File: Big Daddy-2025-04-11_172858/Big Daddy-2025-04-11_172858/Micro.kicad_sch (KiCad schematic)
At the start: 22 parts, among them Q1 2N7002, U1 MAX33054EASA+T, U2 ESP32-S3-DevKitC, U3 ESP32-S3-DevKitC

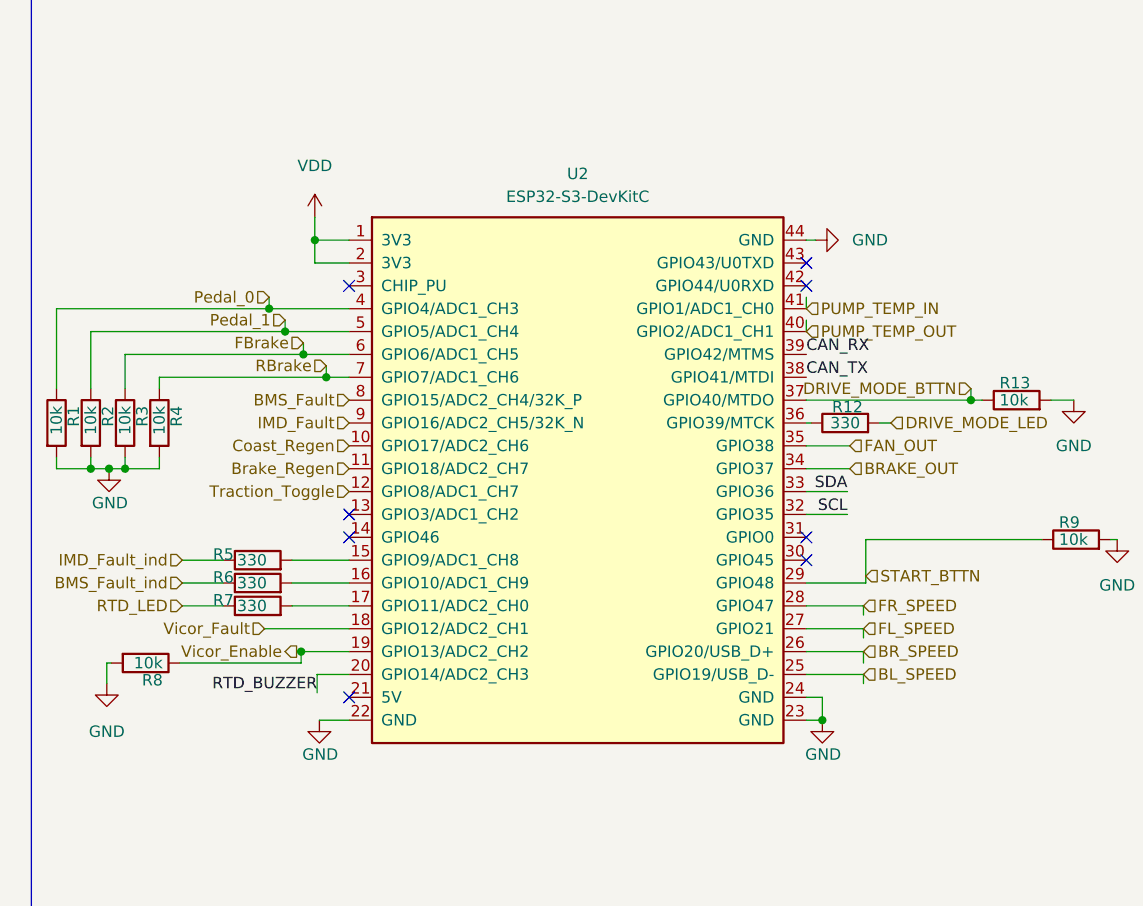
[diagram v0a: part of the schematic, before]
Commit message: all the bs
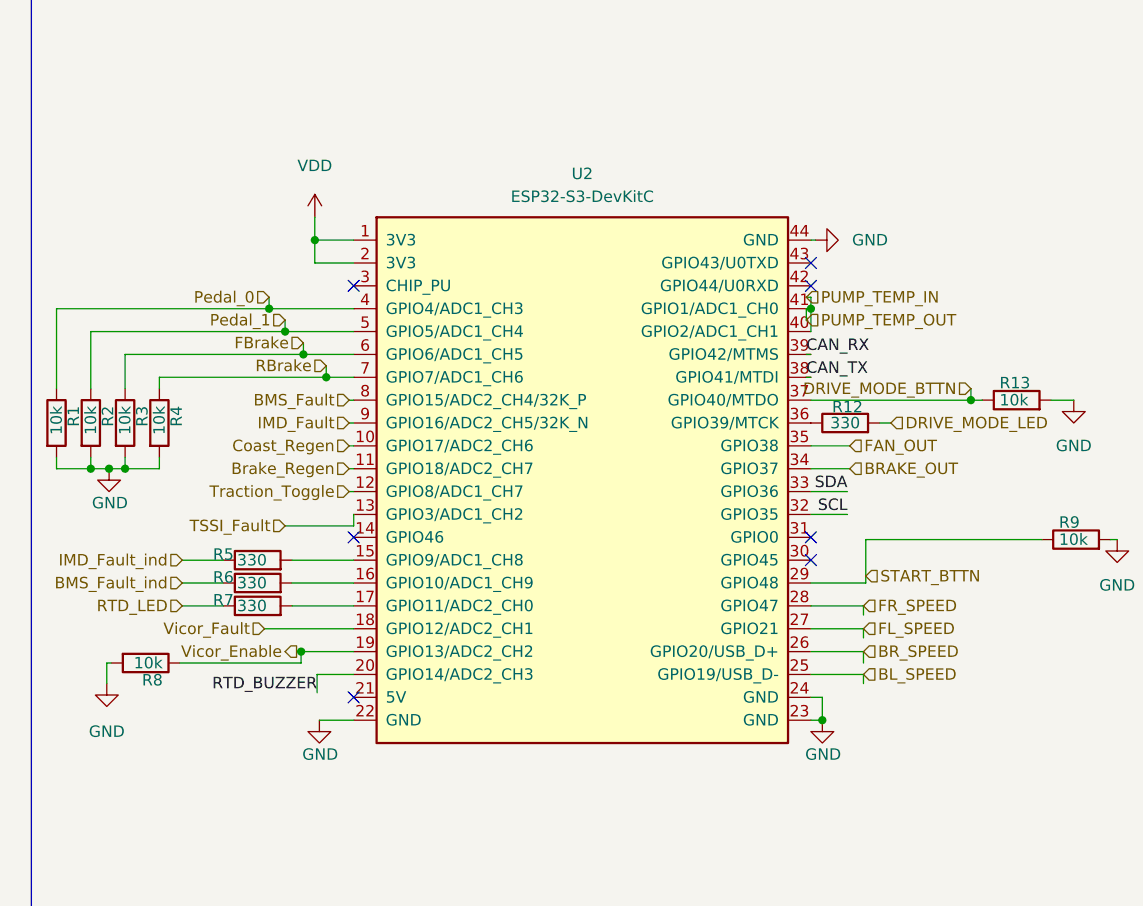
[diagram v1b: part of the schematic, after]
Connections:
- net PUMP_TEMP_OUT is gone; now on net PUMP_TEMP_IN: U2.40 (GPIO2/ADC1_CH1)
- net TSSI_Fault: now reaches U2.13 (GPIO3/ADC1_CH2)
- no-connect marks 19 -> 18
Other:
- moved on the sheet: U2
